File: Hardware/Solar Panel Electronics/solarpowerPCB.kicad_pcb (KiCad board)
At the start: 4 copper layers, 57.8 x 69.2 mm, 157 parts, among them J1 Screw_Terminal_SolarPanel_Inp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, J10 Screw_Terminal_SolarPanel_Inp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, J11 Screw_Terminal_SolarPanel_Inp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, J12 NTC Connector, J13 Battery Connector, J14 Screw_Terminal_5VRail, J2 Screw_Terminal_SolarPanel_Inp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, J3 Conn_01x02_Male, J4 Conn_01x06_Male, J5 Conn_01x02_Male, J6 USB_C_Receptacle_USB2.0, J8 Screw_Terminal_SolarPanel_Inp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, J9 Screw_Terminal_SolarPanel_Inp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, Q1 MMDT2222A, Q2 Q_NMOS_DGS, Q3 Q_NMOS_DGS, U1 SN65HVD230, U2 ESP32-WROOM-32D, U3 LT3652EDD, U4 LTC4411ES5TRMPBF, U5 CP2102-GMR-QFN28, U6 LM5118MH, U7 LT1963AxST-3.3, U8 ADS131M04, U9 ADS1219IPWT

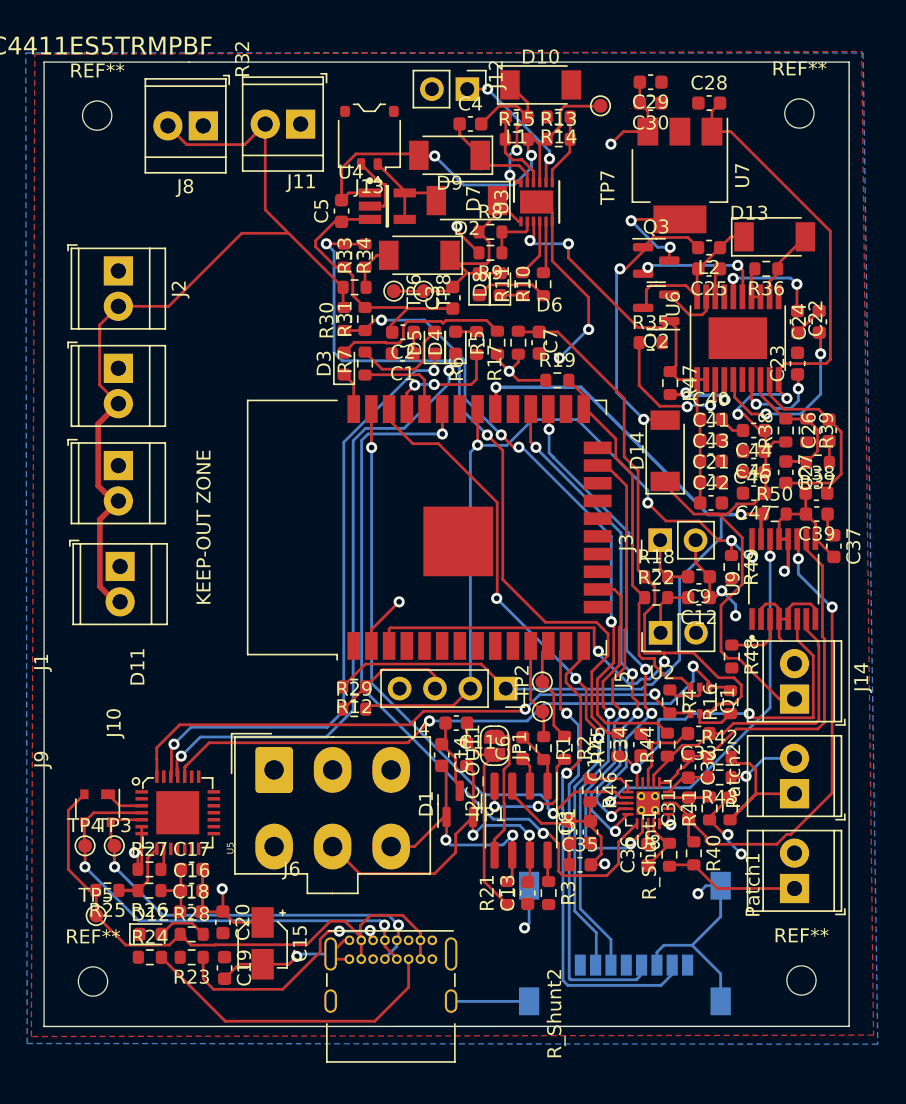
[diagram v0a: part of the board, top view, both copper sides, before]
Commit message: PCB done. Just needs checking
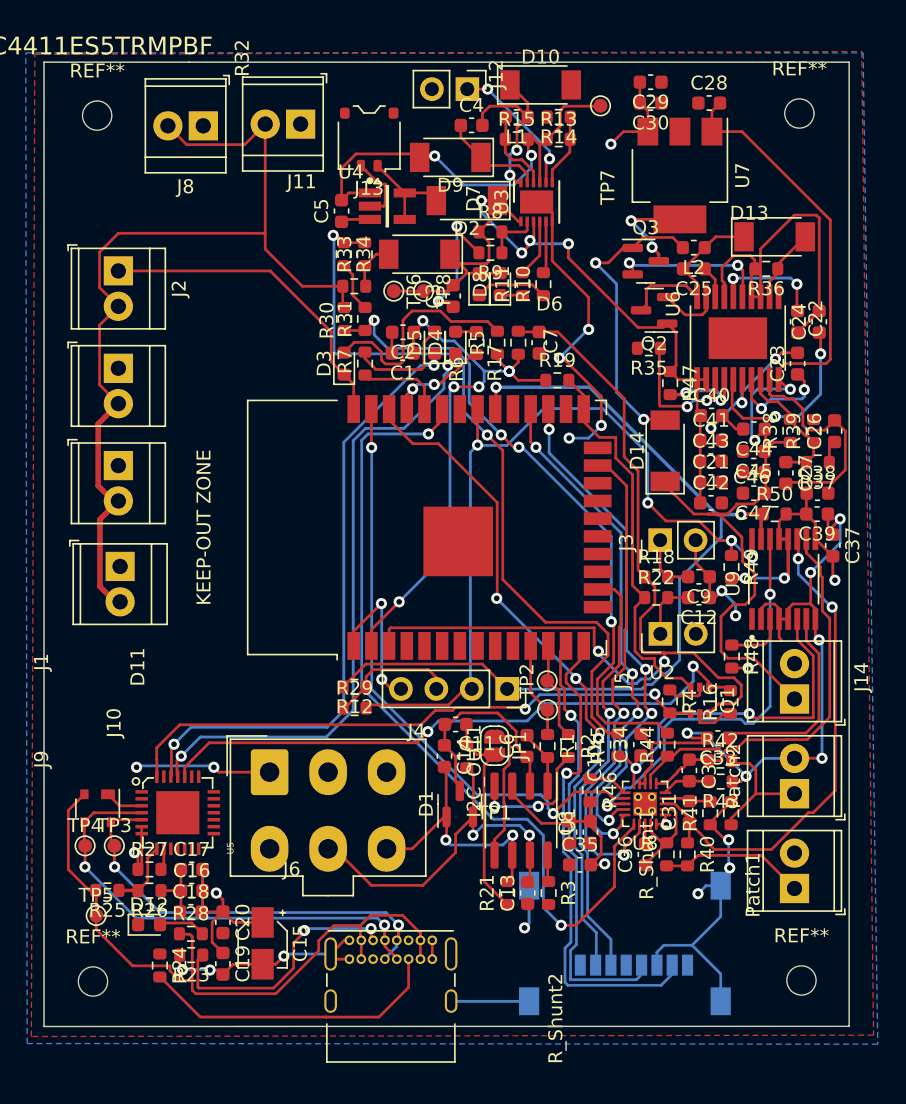
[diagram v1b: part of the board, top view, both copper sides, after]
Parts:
- moved C33 1.41 mm to (74.5, 116.1)
- moved C25 1.09 mm to (72.8, 82.4)
- moved L2 1.09 mm to (72.8, 80.9)
- moved R24 0.93 mm to (34.5, 132.4), turned to -90 degrees
- moved Q3 0.75 mm to (69.3, 81.8)
- moved D12 0.70 mm to (33.7, 129.5)
- moved R39 0.50 mm to (81.4, 94.0), turned to 90 degrees
- moved R40 0.46 mm to (72.3, 124.4)
- moved R35 0.42 mm to (69.6, 88.1), turned to 180 degrees
- moved C26 0.40 mm to (82.9, 94.0)
- moved TP1 0.40 mm to (62.3, 114.0)
- moved J4 0.36 mm to (42.4, 118.5)
- moved TP2 0.36 mm to (62.3, 112.0)
- moved R_Shunt2 0.36 mm to (75.5, 121.5)
- moved R41 0.35 mm to (74.0, 121.5)
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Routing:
- net GND: track 150.7 -> 273.1 mm, vias 13 -> 30
- net +3V3: track 68.3 -> 107.9 mm, vias 8 -> 15
- net VBUS: track 41.8 -> 48.8 mm
- net /VSolCharger: track 51.6 -> 58.5 mm, vias 2 -> 4
- net /VSPI_MOSI: track 54.6 -> 59.4 mm
- net Net-(D3-Pad2): track 13.0 -> 16.2 mm
- net /Solar Charger/V_solarpanel: track 63.8 -> 67.0 mm
- net Net-(Patch2-Pad1): track 11.9 -> 9.45 mm
- net /SCL: track 55.9 -> 58.2 mm
- net /ADC/~{DRDY}: track 27.6 -> 29.6 mm
- net Net-(J6-PadA5): track 16.9 -> 18.7 mm
- net Net-(C26-Pad2): track 14.6 -> 16.3 mm
- net Net-(C25-Pad2): track 11.8 -> 13.5 mm
- net Net-(Q3-Pad2): track 9.53 -> 11.2 mm
- net Net-(R35-Pad1): track 10.9 -> 9.40 mm
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
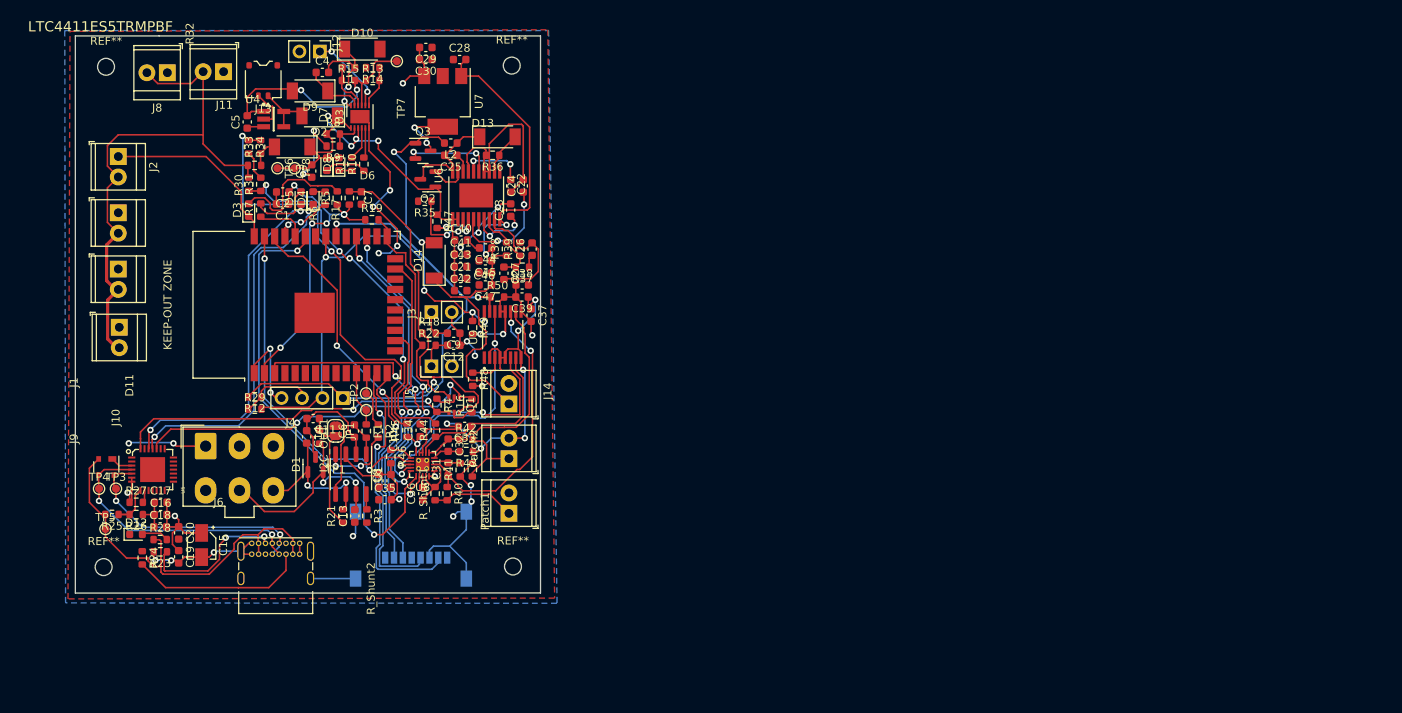
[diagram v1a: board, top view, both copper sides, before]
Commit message: ICARUS v2
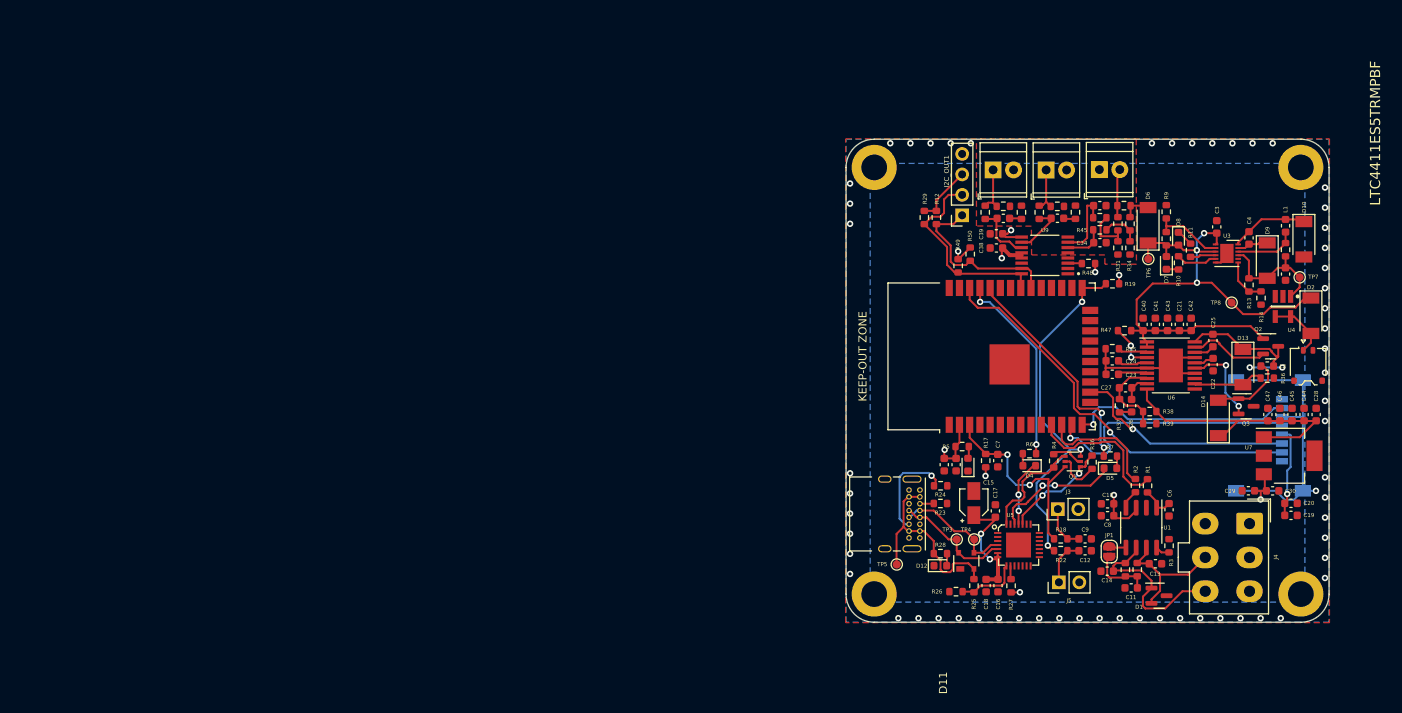
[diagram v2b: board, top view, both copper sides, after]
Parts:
- removed C35, C37: 10uF, Capacitor_SMD:C_0603_1608Metric
- removed C36: 220nF, Capacitor_SMD:C_0603_1608Metric
- removed J10, J11, J2, J8, J9: Screw_Terminal_SolarPanel_Input, TerminalBlock_TE-Connectivity:TerminalBlock_TE_282834-2_1x02_P2.54mm_Horizontal
- removed J12: NTC Connector, Connector_PinHeader_2.54mm:PinHeader_1x02_P2.54mm_Vertical
- removed J14: Screw_Terminal_5VRail, TerminalBlock_TE-Connectivity:TerminalBlock_TE_282834-2_1x02_P2.54mm_Horizontal
- removed R46: 10k, Resistor_SMD:R_0603_1608Metric
- removed the REF** at (29.7, 133.6)
- removed the REF** at (80.5, 133.5)
- removed the REF** at (80.4, 71.2)
- removed the REF** at (30.0, 71.4)
- removed TP1, TP2: TestPoint, TestPoint:TestPoint_Pad_D1.0mm
- removed U8: ADS131M04, Package_DFN_QFN:WQFN-20-1EP_3x3mm_P0.4mm_EP1.7x1.7mm_ThermalVias
- added G***: LOGO, iclr:iclr_logo, B.Cu at (129.0, 92.2)
- added G***: LOGO, iclr:icarus2.0, B.Cu at (149.4, 113.7)
- added REF**: MountingHole_3.2mm_M3_DIN965_Pad, MountingHole:MountingHole_3.2mm_M3_DIN965_Pad, F.Cu at (125.4, 83.9)
- added REF**: MountingHole_3.2mm_M3_DIN965_Pad, MountingHole:MountingHole_3.2mm_M3_DIN965_Pad, F.Cu at (125.4, 136.9)
- added REF**: MountingHole_3.2mm_M3_DIN965_Pad, MountingHole:MountingHole_3.2mm_M3_DIN965_Pad, F.Cu at (178.4, 136.9)
- added REF**: MountingHole_3.2mm_M3_DIN965_Pad, MountingHole:MountingHole_3.2mm_M3_DIN965_Pad, F.Cu at (178.4, 83.9)
- moved C19 138.3 mm to (177.2, 127.1), turned to 0 degrees
- moved C20 138.2 mm to (177.2, 125.6), turned to 0 degrees
- moved J13 134.5 mm to (179.3, 108.5), turned to 0 degrees
- moved C5 130.4 mm to (176.5, 97.2)
- moved J4 130.0 mm to (172.0, 128.2), turned to -90 degrees
- moved U4 127.5 mm to (176.2, 101.2), turned to -90 degrees
- moved D2 125.6 mm to (179.7, 102.3), turned to -90 degrees
- moved J1 122.0 mm to (153.4, 84.2), turned to 0 degrees
- moved D9 120.8 mm to (174.2, 95.5), turned to -90 degrees
- moved D10 119.3 mm to (178.8, 92.8), turned to -90 degrees
- moved R15 118.3 mm to (176.5, 94.1), turned to -90 degrees
- moved L1 118.1 mm to (176.5, 91.2), turned to -90 degrees
- moved C30 118.0 mm to (174.9, 124.1)
- moved TP8 117.6 mm to (169.8, 100.7), turned to 180 degrees
- moved C4 116.9 mm to (172.0, 92.7), turned to 90 degrees
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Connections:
- C33 pad 2: GND -> GNDA
- C34 pad 2: GND -> GNDA
- J1 pad 1: GND -> GNDA
- Patch1 pad 2: GND -> GNDA
- Patch2 pad 2: GND -> GNDA
- R41 pad 1: GND -> GNDA
- R43 pad 1: GND -> GNDA
- R_Shunt1 pad 2: GND -> GNDA
- R_Shunt2 pad 2: GND -> GNDA
- U2 pad 23: /CLKOUT -> unconnected-(U2-Pad23)
- U2 pad 27: /VSPI_SCLK -> unconnected-(U2-Pad27)
- U2 pad 28: /VSPI_MISO -> unconnected-(U2-Pad28)
- U2 pad 33: /VSPI_MOSI -> unconnected-(U2-Pad33)
- U2 pad 37: /~{ADC_CS} -> unconnected-(U2-Pad37)
- U3 pad 8: Net-(J12-Pad1) -> unconnected-(U3-Pad8)
- U6 pad 21: unconnected-(U6-Pad21) -> GND
- U9 pad 5: GND -> GNDA
- U9 pad 8: GND -> GNDA
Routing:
- net GND: track 273.1 -> 59.9 mm, vias 30 -> 62
- net /Solar Charger/V_solarpanel: track 67.0 -> 6.06 mm
- net /VSPI_MOSI: track 59.4 -> 0.00 mm, vias 2 -> 0
- net /SolarPanelVoltage2: track 55.1 -> 4.84 mm, vias 2 -> 0
- net /~{ADC_CS}: track 43.1 -> 0.00 mm, vias 2 -> 0
- net /SDA: track 64.5 -> 22.0 mm, vias 2 -> 0
- net /SolarPanelVoltage1: track 47.1 -> 6.12 mm, vias 4 -> 0
- net /EN: track 67.3 -> 26.4 mm
- net +3V3: track 107.9 -> 67.7 mm, vias 15 -> 13
- net /VoltageReg/V_reg: track 72.3 -> 34.1 mm, vias 2 -> 0
- net /VSPI_MISO: track 37.8 -> 0.00 mm, vias 4 -> 0
- net /RXD: track 45.5 -> 8.32 mm
- net /VSPI_SCLK: track 36.5 -> 0.00 mm, vias 4 -> 0
- net /CLKOUT: track 36.0 -> 0.00 mm, vias 2 -> 0
- net /SCL: track 58.2 -> 25.0 mm, vias 4 -> 0
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- added copper zone on B.Cu, net GND
- added copper zone on F.Cu, net GNDA
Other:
- board size 57.8 x 69.2 mm -> 60 x 60 mm
- copper layers 4 -> 2
- board text added: "Designed By: Gabisanth Seyon Danielle Bella Artem Sheykin"
- board text added: "I - Imperial C - College A - Avionics R - Run U - Using S - Solar power"
- board text added: "ICARUS v2.0"
